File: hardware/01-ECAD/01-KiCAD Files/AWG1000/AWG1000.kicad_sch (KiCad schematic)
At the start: 0 parts

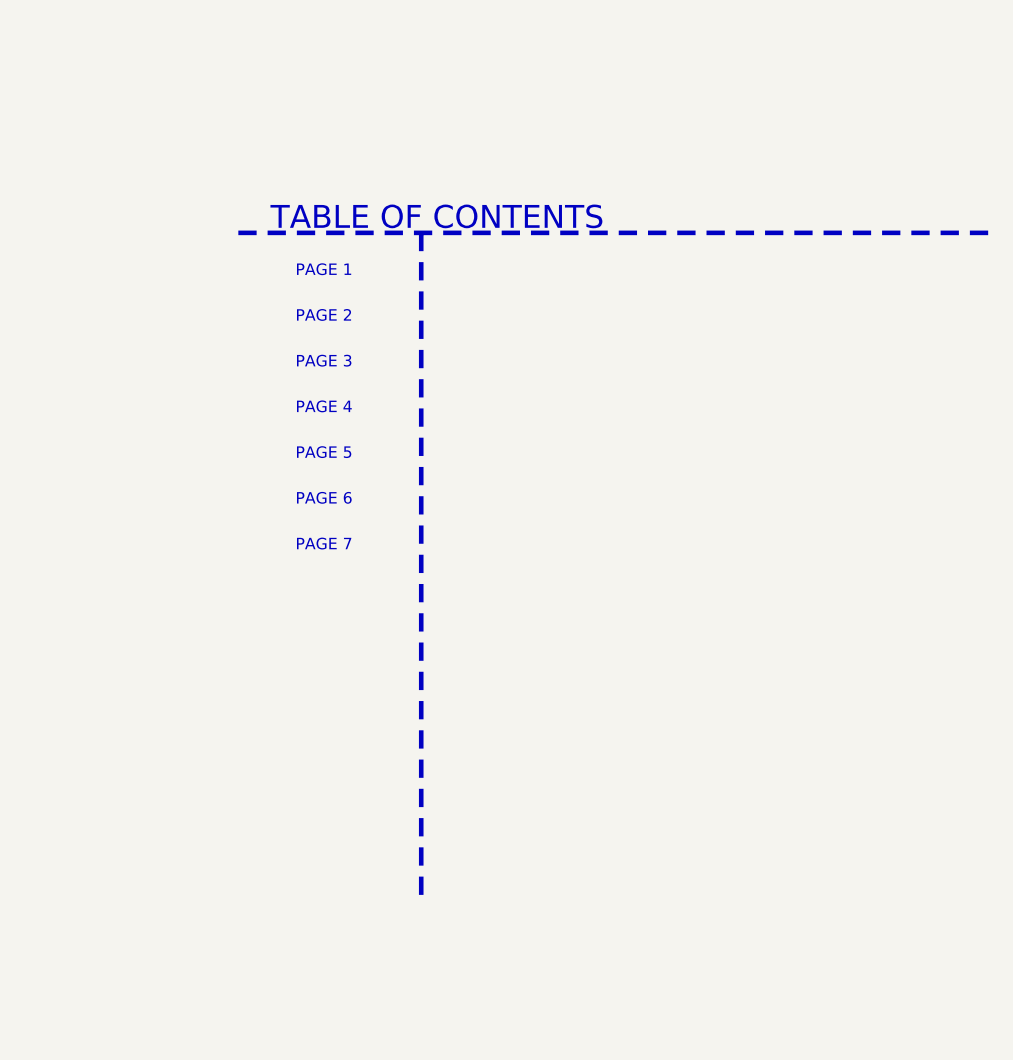
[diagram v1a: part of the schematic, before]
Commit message: Update.
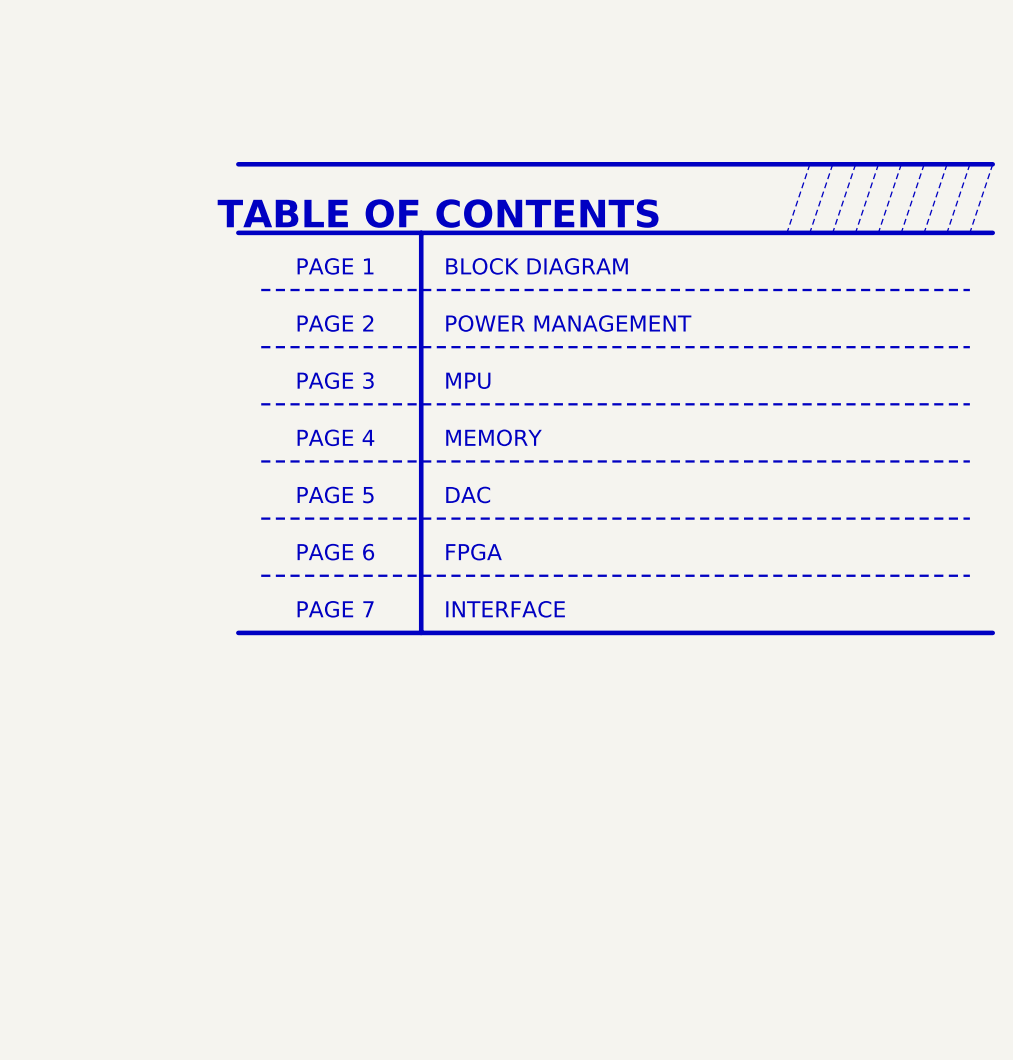
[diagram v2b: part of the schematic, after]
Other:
- note added: "BLOCK DIAGRAM"
- note added: "DAC"
- note added: "FPGA"
- note added: "INTERFACE"
- note added: "MEMORY"
- note added: "MPU"
- note added: "POWER MANAGEMENT"
- title: (none) -> AWG100 MB
